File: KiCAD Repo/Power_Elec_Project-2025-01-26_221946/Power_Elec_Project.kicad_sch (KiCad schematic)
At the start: 0 parts

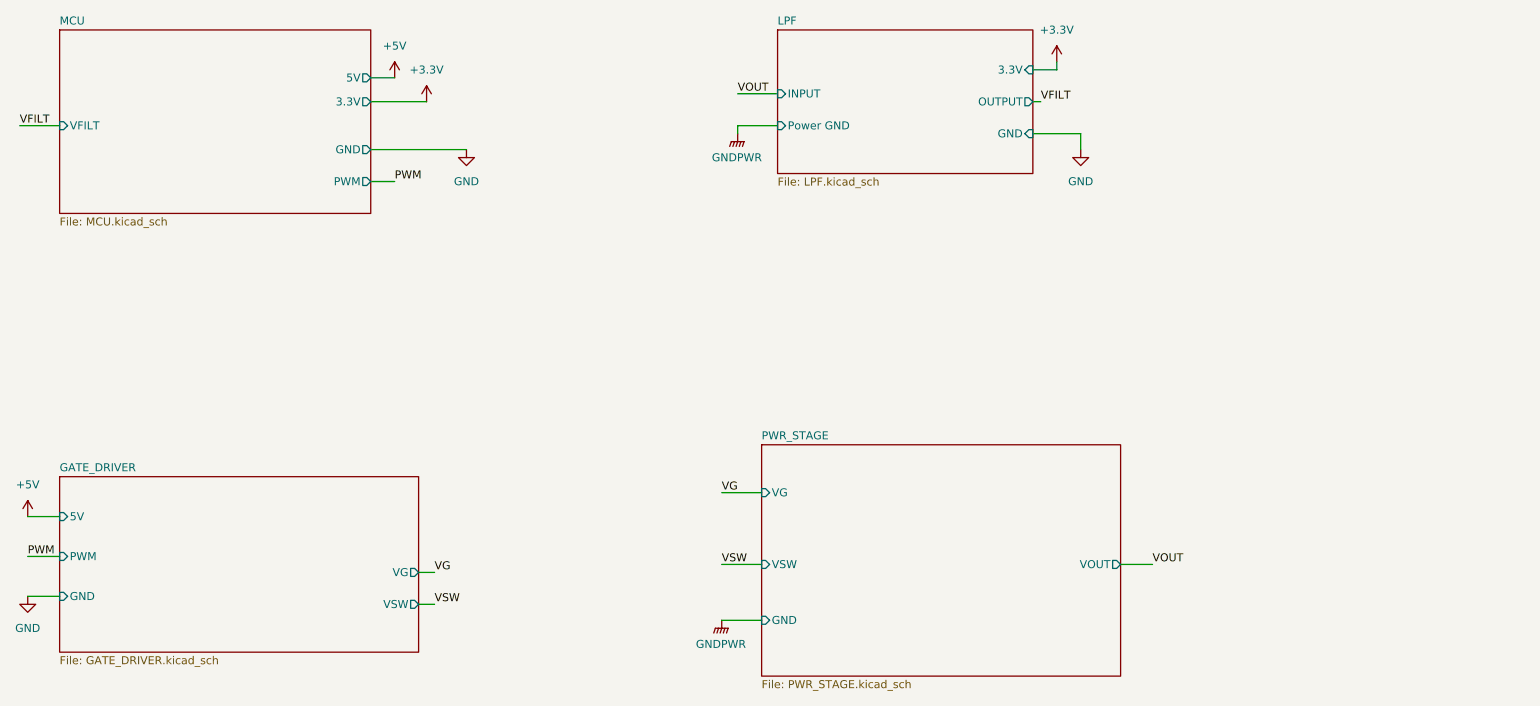
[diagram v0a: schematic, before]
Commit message: PCB fix
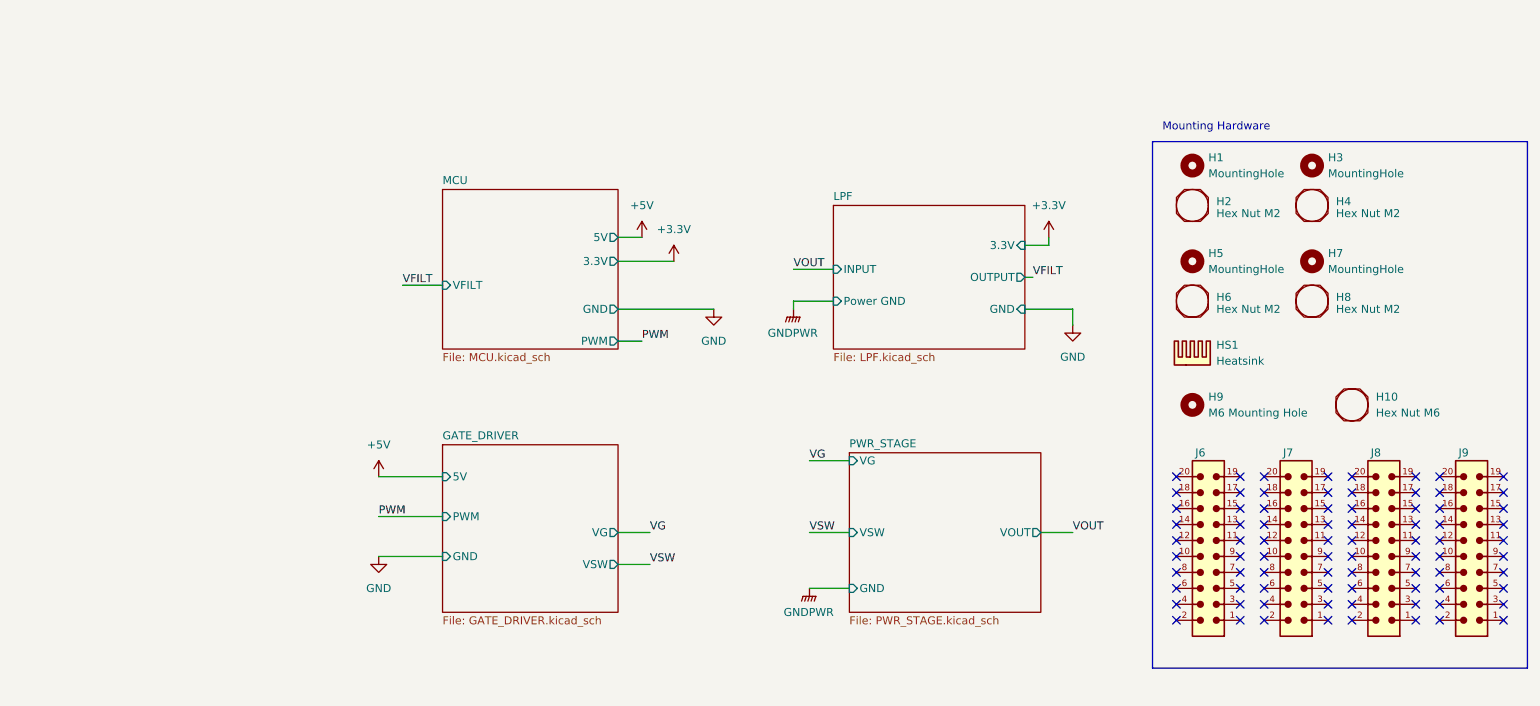
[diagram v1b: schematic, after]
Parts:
- added H1, H3, H5, H7: MountingHole, MountingHole:MountingHole_2.2mm_M2, symbol Mechanical:MountingHole
- added H10: Hex Nut M6, ~, symbol Uwindsor:Mounting_Nut
- added H2, H4, H6, H8: Hex Nut M2, ~, symbol Uwindsor:Mounting_Nut
- added H9: M6 Mounting Hole, MountingHole:MountingHole_6.4mm_M6, symbol Mechanical:MountingHole
- added HS1: Heatsink, Heatsink:Heatsink_Stonecold_HS-S03_13.21x12.7mm, symbol Mechanical:Heatsink
- added J6, J7, J8, J9: 6120XX21621, 6120XX21621_61202021621:61202021621, symbol Connector_Launchpad_61202021621:6120XX21621_61202021621
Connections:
- no-connect marks 0 -> 80
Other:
- note added: "Mounting Hardware"
